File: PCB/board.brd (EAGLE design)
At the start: 35 x 48.5 mm, 9 parts, among them J1 PROG-HEADER_2X3_SHROUDED, J10 PROG-HEADER_2X5_1.27MM-SHROUD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, J2 PROG-HEADER_2X5_2.00MM-SHROUD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, J3 PROG-HEADER_2X5_SHROUDED, J4 PROG-HEADER_2X10_2.54MM-END-L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, J6 PROG-HEADER_2X10_SHROUDED, J8 CONN-1X4, J9 CONN-1X6

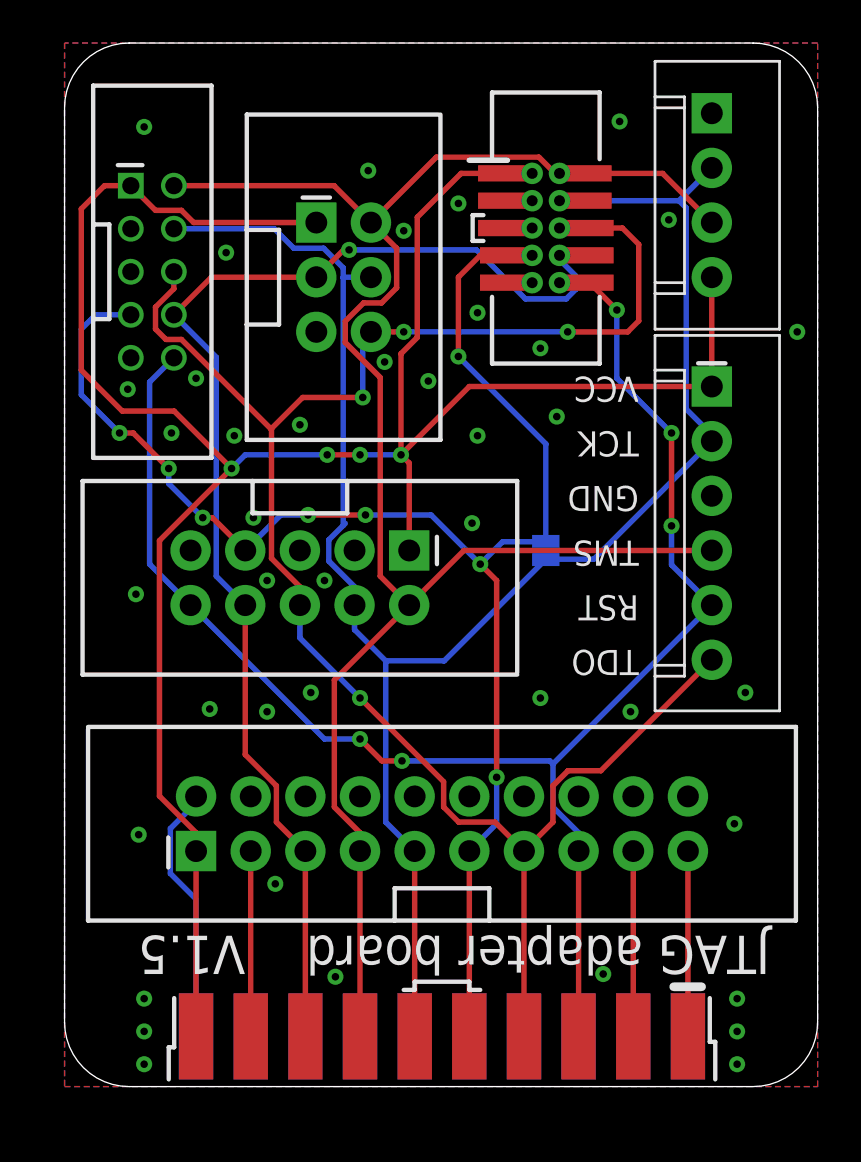
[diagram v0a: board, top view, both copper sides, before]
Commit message: rollback to V1.4
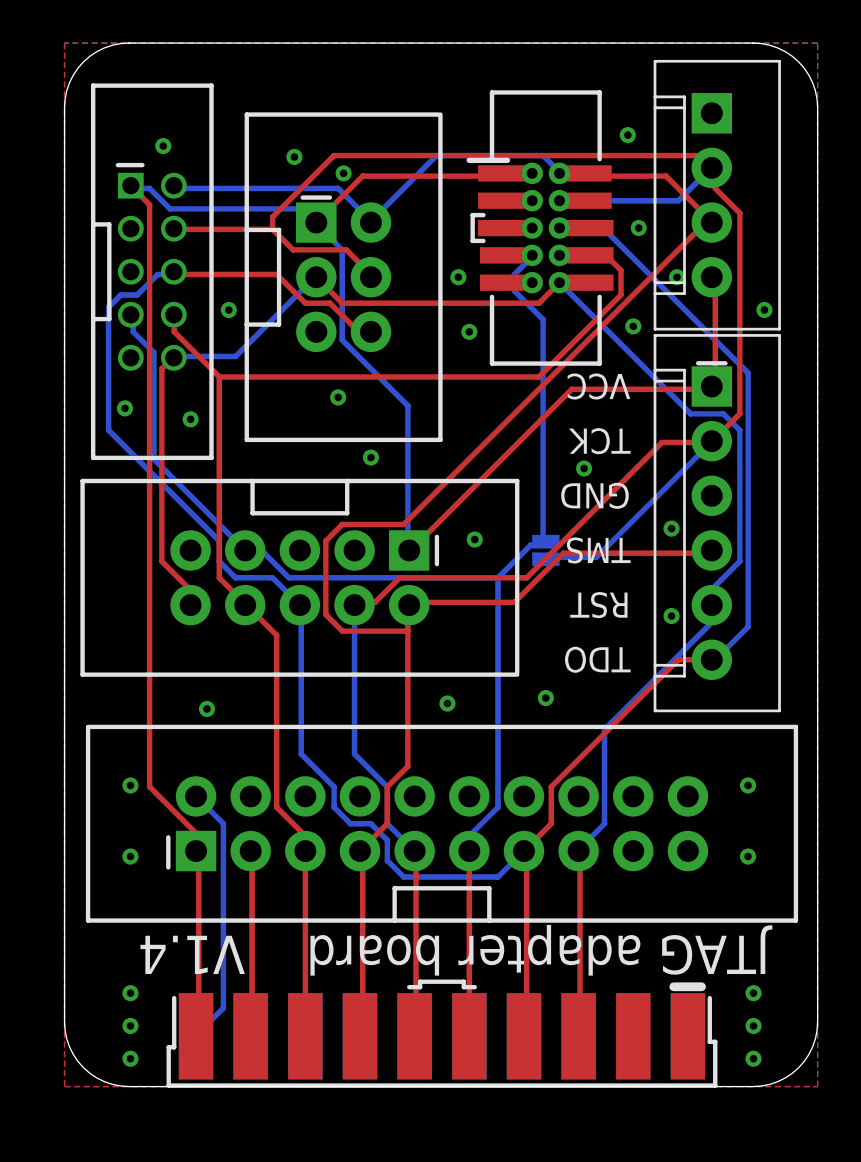
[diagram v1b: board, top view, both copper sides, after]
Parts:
- JP1: device angrypig7-Jumpers:SMT-JUMPER_2_NO_SILK -> SparkFun-Jumpers:SMT-JUMPER_2_NO_SILK
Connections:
- net VREF renamed VCC
- removed net 17: J4.17, J6.17
- removed net 19: J4.19, J6.19
- net RST: now also J1.3
- net TDI: no longer J1.3
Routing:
- net TCK: track 86.6 -> 106.5 mm
- net TDO: track 84.8 -> 103.2 mm, vias 4 -> 0
- net TMS: track 85.1 -> 96.4 mm
- net 19: track 8.61 -> 0.00 mm
- net 17: track 8.61 -> 0.00 mm
- net RTCK: track 72.1 -> 65.8 mm, vias 8 -> 0
- net VCC: track 106.7 -> 100.8 mm, vias 4 -> 0
- net RST: track 73.7 -> 76.5 mm, vias 5 -> 0
- net TDI: track 59.0 -> 60.7 mm, vias 1 -> 0

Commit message: V1.6 update
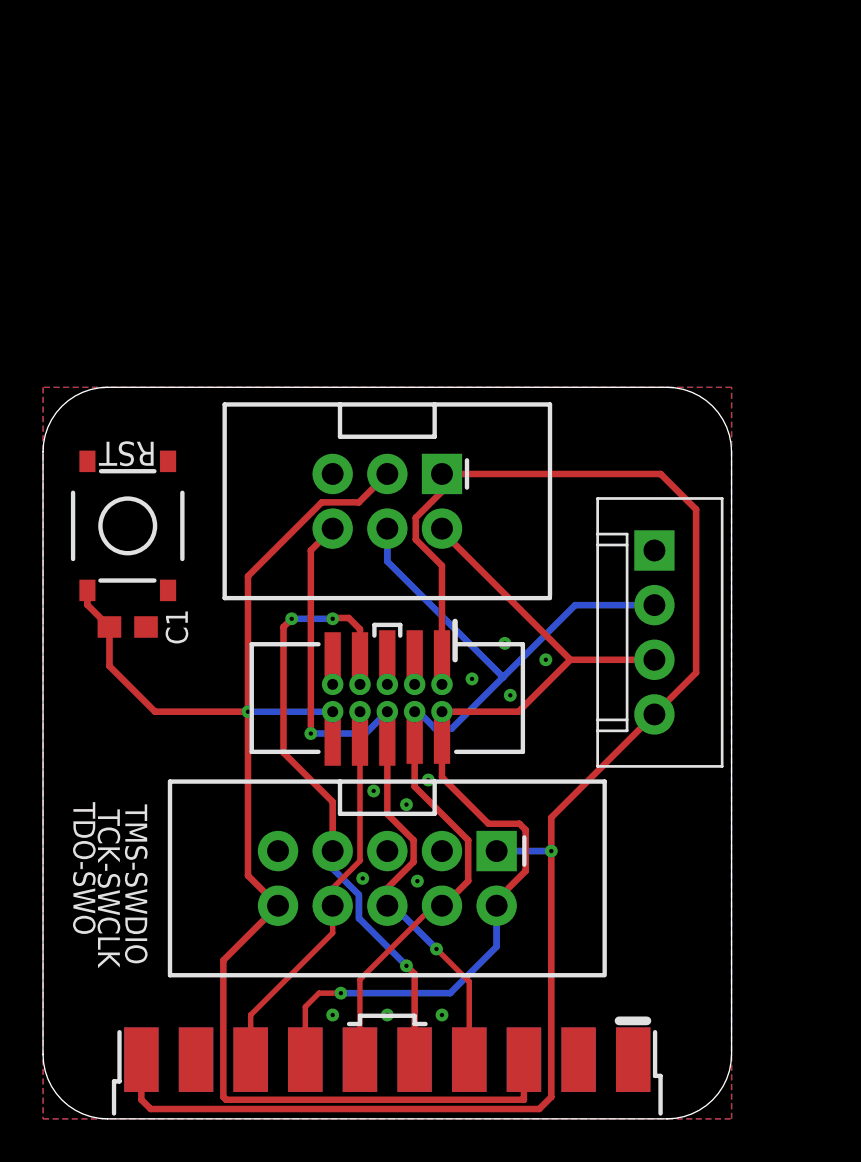
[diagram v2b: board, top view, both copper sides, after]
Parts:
- removed J2: PROG-HEADER_2X5_2.00MM-SHROUDED, angrypig7-Connectors-Programming:2X5-2.00MM-SHROUDED
- removed J6: PROG-HEADER_2X10_SHROUDED, angrypig7-Connectors-Programming:2X10-2.54MM-SHROUDED
- removed J9: CONN-1X6, angrypig7-Connectors-Programming:MOLEX-1X6-2.54MM
- removed JP1: TCK-RTCK, SparkFun-Jumpers:SMT-JUMPER_2_NO_SILK
- added C1: 100nF, angrypig7-RCL:C0603
- added S1: SWITCH-SPST-SMD-5.1MM, angrypig7-Switches:TACTILE_SWITCH_SMD_5.1MM
- J8: device angrypig7-Connectors-Programming:MOLEX-1X4-2.54MM -> angrypig7-Connectors-Programming:XH-4P-2.54MM
- moved J8 24.3 mm to (28.4, 22.6)
- moved J10 23.1 mm to (16.0, 19.6), turned to 180 degrees
- moved J3 14.5 mm to (16.0, 11.2)
- moved J1 10.6 mm to (16.0, 28.7), turned to 270 degrees
- moved J4 3.00 mm to (16.0, 2.25)
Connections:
- net 2: no longer J6.2
- net GND: now also C1.2, S1.3; no longer J2.3, J2.5, J2.9, J6.10, J6.12, J6.14, J6.16, J6.18, J6.20, J6.4, J6.6, J6.8, J9.3
- net NTRST: no longer J6.3
- net RST: now also C1.1, S1.1; no longer J2.10, J6.15, J9.5
- net RTCK: no longer J2.7, J6.11, JP1.2
- net TCK: no longer J2.4, J6.9, J9.2, JP1.1
- net TDI: no longer J2.8, J6.5
- net TDO: no longer J2.6, J6.13, J9.6
- net TMS: no longer J2.2, J6.7, J9.4
- net VCC: no longer J2.1, J6.1, J9.1
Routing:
- net TDO: track 103.2 -> 31.5 mm, vias 0 -> 2
- net TCK: track 106.5 -> 41.3 mm
- net TMS: track 96.4 -> 44.7 mm, vias 0 -> 1
- net TDI: track 60.7 -> 17.0 mm
- net RTCK: track 65.8 -> 27.9 mm, vias 0 -> 3
- net VCC: track 100.8 -> 75.9 mm, vias 0 -> 1
- net 2: track 12.2 -> 0.00 mm
- net RST: track 76.5 -> 65.4 mm, vias 0 -> 1
- net NTRST: track 8.65 -> 0.00 mm
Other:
- board size 35 x 48.5 mm -> 32 x 34 mm
- board text removed: ">CREVISION"
- board text removed: ">GITHUB"
- board text removed: "TCK-RTCK"
